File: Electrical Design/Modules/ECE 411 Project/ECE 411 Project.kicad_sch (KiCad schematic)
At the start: 48 parts, among them J1 5mm 9V Barrel, J2 BOOST, J3 Pheonix Connector, J4 1/8in Jack, J5 1x2 header, J6 1x2header, J7 1x2header, SW1 SW_Push, SW10 SW_SPDT, SW2 SW_Push, SW3 SW_Push, SW4 SW_Push, SW5 SW_Push, SW6 SW_Push, SW7 SW_Push, SW9 SW_SPDT, U1 HT7333, U2 LT1054

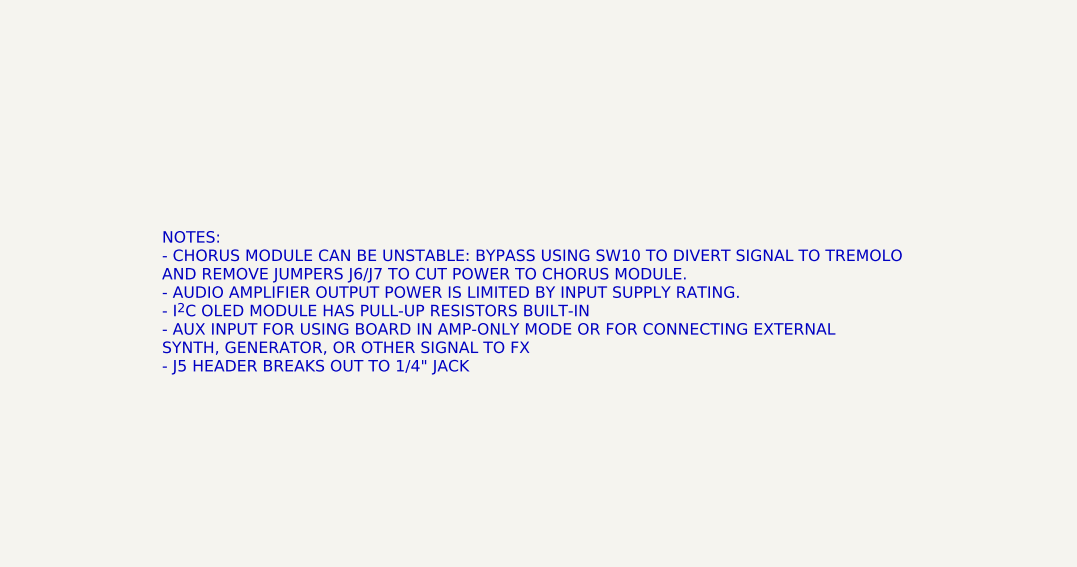
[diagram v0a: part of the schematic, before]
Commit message: pcb finalization
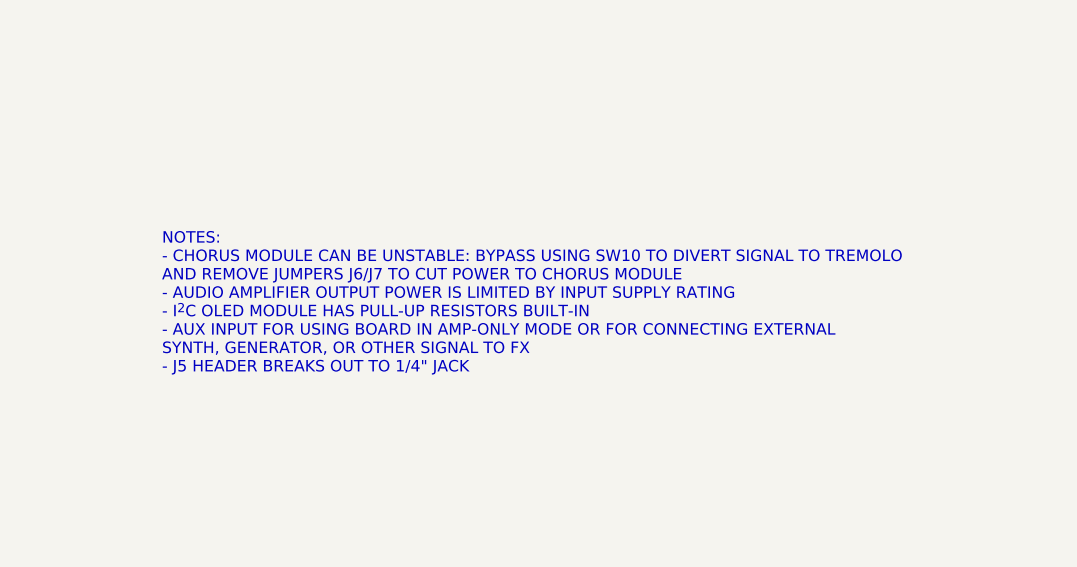
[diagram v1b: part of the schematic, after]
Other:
- note added: "NOTES: - CHORUS MODULE CAN BE UNSTABLE: BYPASS USING SW10 TO DIVERT SIGNAL TO TREMOLO AND REMOVE JUMPERS J6/J7 TO CUT POWER TO CHORUS MODULE - AUDIO AMPLIFIER OUTPUT POWER IS LIMITED BY INPUT SUPPLY RATING - I^{2}C OLED MODULE HAS PULL-UP RESISTORS BUILT-IN - AUX INPUT FOR USING BOARD IN AMP-ONLY MODE OR FOR CONNECTING EXTERNAL SYNTH, GENERATOR, OR OTHER SIGNAL TO FX - J5 HEADER BREAKS OUT TO 1/4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"
- note removed: "NOTES: - CHORUS MODULE CAN BE UNSTABLE: BYPASS USING SW10 TO DIVERT SIGNAL TO TREMOLO AND REMOVE JUMPERS J6/J7 TO CUT POWER TO CHORUS MODULE. - AUDIO AMPLIFIER OUTPUT POWER IS LIMITED BY INPUT SUPPLY RATING. - I^{2}C OLED MODULE HAS PULL-UP RESISTORS BUILT-IN - AUX INPUT FOR USING BOARD IN AMP-ONLY MODE OR FOR CONNECTING EXTERNAL SYNTH, GENERATOR, OR OTHER SIGNAL TO FX - J5 HEADER BREAKS OUT TO 1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"
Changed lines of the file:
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@@
 		)
 	)
-	(text "NOTES:\n- CHORUS MODULE CAN BE UNSTABLE: BYPASS USING SW10 TO DIVERT SIGNAL TO TREMOLO\nAND REMOVE JUMPERS J6/J7 TO CUT POWER TO CHORUS MODULE.\n- AUDIO AMPLIFIER OUTPUT POWER IS LIMITED BY INPUT SUPPLY RATING.\n- I^{2}C OLED MODULE HAS PULL-UP RESISTORS BUILT-IN\n- AUX INPUT FOR USING BOARD IN AMP-ONLY MODE OR FOR CONNECTING EXTERNAL\nSYNTH, GENERATOR, OR OTHER SIGNAL TO FX\n- J5 HEADER BREAKS OUT TO 1/4\" JACK"
+	(text "NOTES:\n- CHORUS MODULE CAN BE UNSTABLE: BYPASS USING SW10 TO DIVERT SIGNAL TO TREMOLO\nAND REMOVE JUMPERS J6/J7 TO CUT POWER TO CHORUS MODULE\n- AUDIO AMPLIFIER OUTPUT POWER IS LIMITED BY INPUT SUPPLY RATING\n- I^{2}C OLED MODULE HAS PULL-UP RESISTORS BUILT-IN\n- AUX INPUT FOR USING BOARD IN AMP-ONLY MODE OR FOR CONNECTING EXTERNAL\nSYNTH, GENERATOR, OR OTHER SIGNAL TO FX\n- J5 HEADER BREAKS OUT TO 1/4\" JACK"
 		(exclude_from_sim no)
 		(at 177.8 151.765 0)

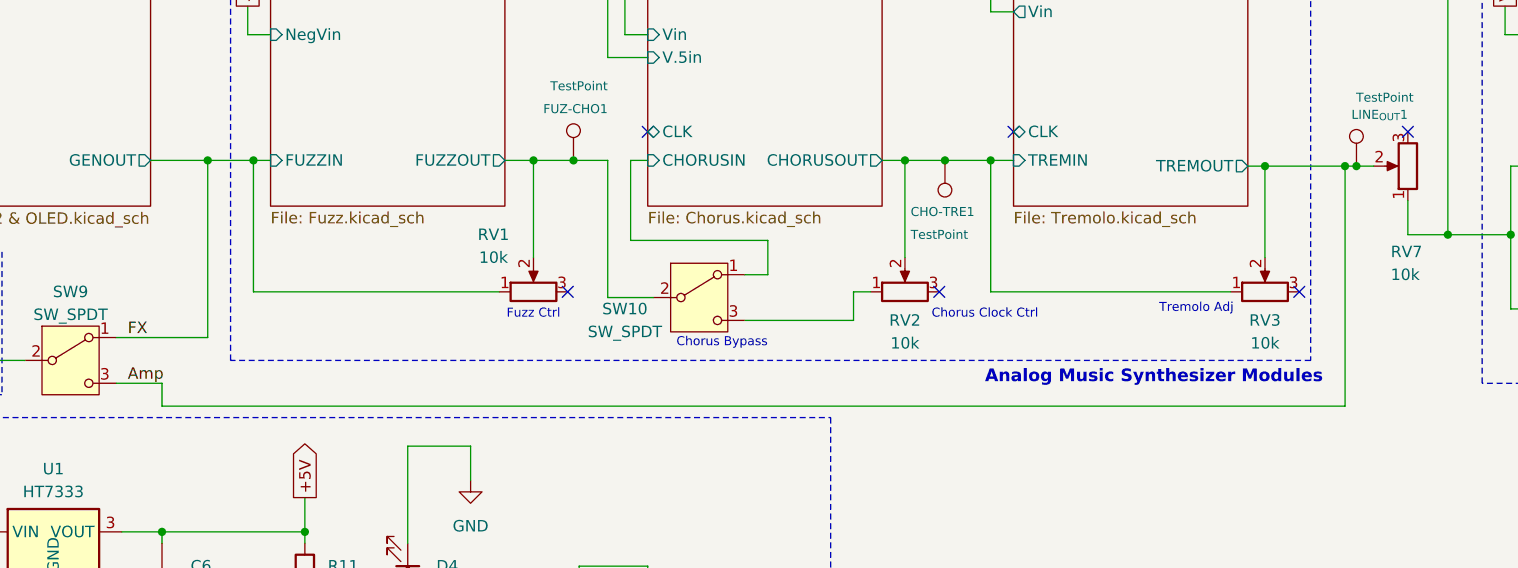
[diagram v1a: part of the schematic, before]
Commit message: pcb madness
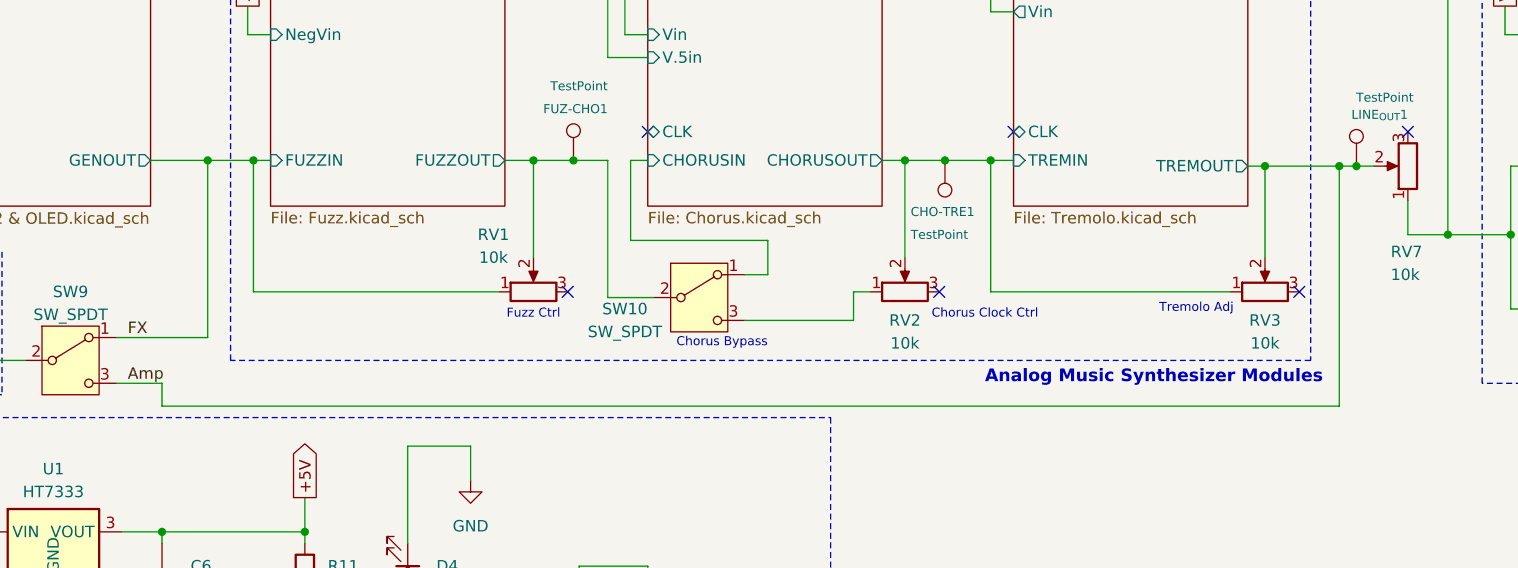
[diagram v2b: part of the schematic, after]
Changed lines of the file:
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@@
-	)
-	(junction
-		(at 203.2 79.375)
-		(diameter 0)
-		(color 0 0 0 0)
 	)
 	(junction
@@
 	(junction
 		(at 34.29 140.97)
+		(diameter 0)
+		(color 0 0 0 0)
+	)
+	(junction
+		(at 202.565 79.375)
 		(diameter 0)
 		(color 0 0 0 0)
@@
 	(wire
 		(pts
-			(xy 204.47 79.375) (xy 203.2 79.375)
-		)
-		(stroke
-			(width 0)
-			(type default)
-		)
-	)
-	(wire
-		(pts
 			(xy 99.06 110.49) (xy 106.045 110.49)
 		)
@@
 	(wire
 		(pts
-			(xy 194.31 79.375) (xy 203.2 79.375)
+			(xy 194.31 79.375) (xy 202.565 79.375)
 		)
 		(stroke
@@
 	(wire
 		(pts
-			(xy 71.755 106.045) (xy 203.2 106.045)
+			(xy 71.755 106.045) (xy 202.565 106.045)
 		)
 		(stroke
@@
 	(wire
 		(pts
-			(xy 203.2 106.045) (xy 203.2 79.375)
+			(xy 202.565 106.045) (xy 202.565 79.375)
 		)
 		(stroke
@@
 		)
 		(stroke
+			(width 0)
+			(type default)
+		)
+	)
+	(wire
+		(pts
+			(xy 202.565 79.375) (xy 204.47 79.375)
+		)
+		(stroke
